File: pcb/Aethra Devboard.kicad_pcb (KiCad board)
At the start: 2 copper layers, 21 x 51 mm, 44 parts, among them J1 USB_C_Receptacle_USB2.0_14P, J2 Conn_01x20, J3 Conn_01x20, J4 Conn_01x03, J5 Conn_01x02, Q1 DMG2301L, SW1 SW_Push, U1 RP2040, U2 AP2112K-3.3, U3 W25Q16JVZPIQ, U4 MCP73831-2-OT, Y1 12 MHz

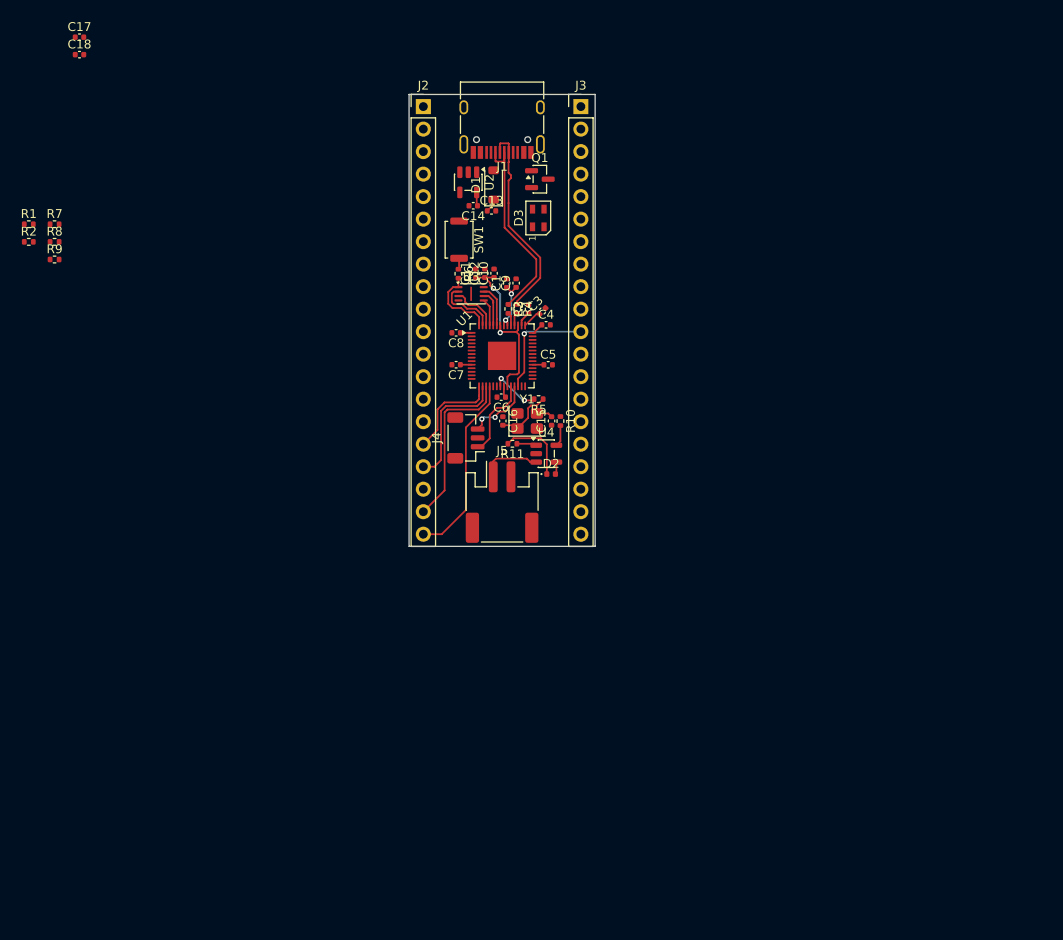
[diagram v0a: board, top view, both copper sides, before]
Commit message: Finish routing PCB
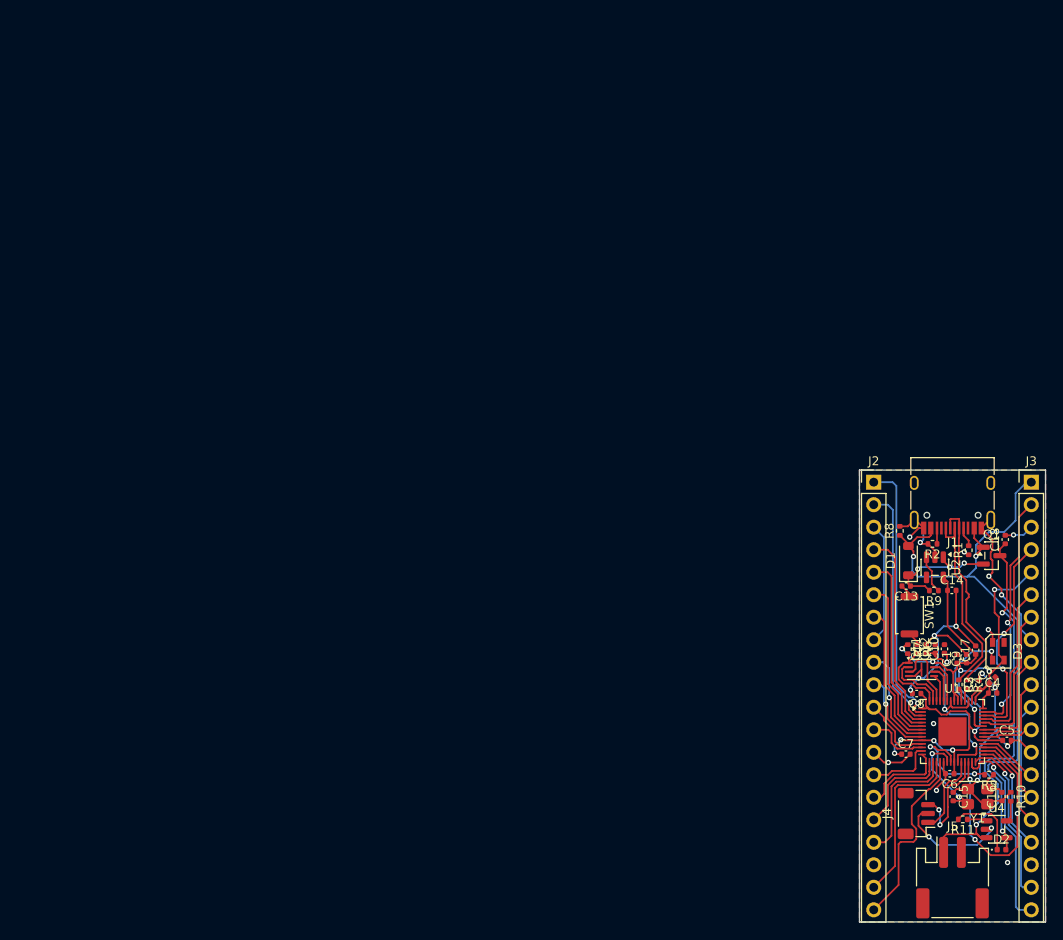
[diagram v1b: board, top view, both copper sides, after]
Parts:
- moved C17 122.5 mm to (153.2, 98.4), turned to 90 degrees
- moved C18 117.9 mm to (156.6, 86.0), turned to 90 degrees
- moved R1 112.3 mm to (152.4, 87.2), turned to 90 degrees
- moved R7 107.6 mm to (145.6, 98.3), turned to -90 degrees
- moved R2 107.5 mm to (148.4, 86.4), turned to 180 degrees
- moved R9 106.0 mm to (148.5, 91.7), turned to 180 degrees
- moved R8 100.8 mm to (144.7, 85.0), turned to 90 degrees
- moved D3 71.3 mm to (155.8, 98.6), turned to -90 degrees
- moved C16 70.5 mm to (156.2, 115.0), turned to 90 degrees
- moved C14 69.3 mm to (150.6, 91.7), turned to 0 degrees
- moved U2 68.3 mm to (148.6, 89.1)
- moved C7 67.1 mm to (145.4, 110.2), turned to 0 degrees
- moved C5 66.9 mm to (156.8, 108.6)
- moved R6 66.9 mm to (146.6, 98.3)
- moved Q1 66.4 mm to (155.0, 87.8)
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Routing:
- net GND: track 0.00 -> 127.6 mm, vias 0 -> 21
- net +3V3: track 17.7 -> 95.6 mm, vias 2 -> 10
- net VBUS: track 1.39 -> 71.4 mm, vias 0 -> 3
- net +BATT: track 6.89 -> 46.2 mm, vias 0 -> 2
- net GPIO0: track 0.00 -> 30.5 mm, vias 0 -> 1
- net GPIO1: track 0.00 -> 27.7 mm, vias 0 -> 1
- net GPIO29_ADC3: track 0.00 -> 27.6 mm, vias 0 -> 2
- net GPIO28_ADC2: track 0.00 -> 23.7 mm, vias 0 -> 2
- net GPIO2: track 0.00 -> 22.9 mm
- net GPIO16: track 0.00 -> 22.7 mm, vias 0 -> 1
- net GPIO3: track 0.00 -> 20.8 mm
- net GPIO17: track 0.00 -> 19.0 mm, vias 0 -> 1
- net RUN: track 12.7 -> 31.4 mm, vias 1 -> 3
- net GPIO4: track 0.00 -> 18.6 mm
- net GPIO27_ADC1: track 0.00 -> 18.3 mm
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- added copper zone on B.Cu, net GND
- added copper zone on F.Cu, net GND
